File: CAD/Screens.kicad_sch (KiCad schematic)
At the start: 2 parts, among them J7 RoundDisplay_SPI, J9 RoundDisplay_SPI_v2

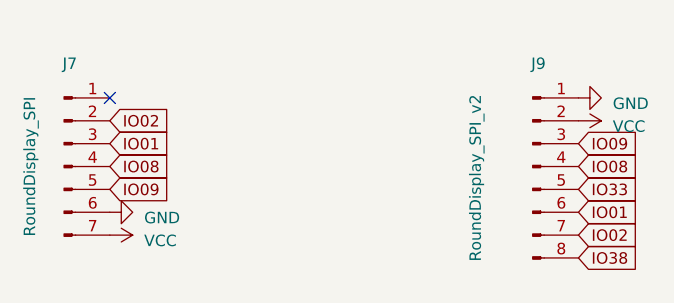
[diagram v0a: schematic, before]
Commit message: Updated pins and moar
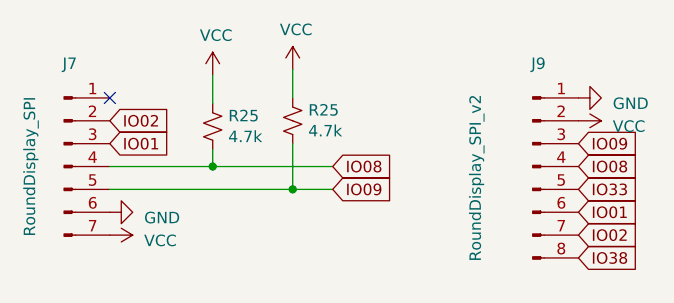
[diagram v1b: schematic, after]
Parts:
- added R25 (x2): 4.7k, BadgePirates:R_1206_3216Metric, symbol Device:R_Small_US
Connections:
- net IO08: now also R25.2
- net IO09: now also R25.2
- net VCC: now also R25.1, R25.1
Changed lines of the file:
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@@
 (kicad_sch (version 20230121) (generator eeschema)
   (paper "A4")
+  (junction (at 153.67 80.01) (diameter 0) (color 0 0 0 0)
+  )
+  (junction (at 144.78 77.47) (diameter 0) (color 0 0 0 0)
+  )
   (no_connect (at 133.35 69.85))
+  (wire (pts (xy 153.67 66.675) (xy 153.67 69.85))
+    (stroke (width 0) (type default))
+  )
+  (wire (pts (xy 144.78 75.565) (xy 144.78 77.47))
+    (stroke (width 0) (type default))
+  )
+  (wire (pts (xy 153.67 74.93) (xy 153.67 80.01))
+    (stroke (width 0) (type default))
+  )
+  (wire (pts (xy 144.78 67.31) (xy 144.78 70.485))
+    (stroke (width 0) (type default))
+  )
+  (wire (pts (xy 153.67 80.01) (xy 133.35 80.01))
+    (stroke (width 0) (type default))
+  )
+  (wire (pts (xy 158.115 80.01) (xy 153.67 80.01))
+    (stroke (width 0) (type default))
+  )
+  (wire (pts (xy 144.78 77.47) (xy 133.35 77.47))
+    (stroke (width 0) (type default))
+  )
+  (wire (pts (xy 158.115 77.47) (xy 144.78 77.47))
+    (stroke (width 0) (type default))
+  )
   (global_label "IO02" (shape input) (at 133.35 72.39 0) (fields_autoplaced)
     (effects (font (size 1.27 1.27)) (justify left))
@@
     )
   )
-  (global_label "IO08" (shape input) (at 133.35 77.47 0) (fields_autoplaced)
-    (effects (font (size 1.27 1.27)) (justify left))
-    (property "Intersheetrefs" "${INTERSHEET_REFS}" (at 139.9559 77.47 0)
+  (global_label "IO08" (shape input) (at 158.115 77.47 0) (fields_autoplaced)
+    (effects (font (size 1.27 1.27)) (justify left))
+    (property "Intersheetrefs" "${INTERSHEET_REFS}" (at 164.7209 77.47 0)
       (effects (font (size 1.27 1.27)) (justify left) hide)
     )
@@
     )
   )
-  (global_label "IO09" (shape input) (at 133.35 80.01 0) (fields_autoplaced)
-    (effects (font (size 1.27 1.27)) (justify left))
-    (property "Intersheetrefs" "${INTERSHEET_REFS}" (at 139.9559 80.01 0)
+  (global_label "IO09" (shape input) (at 158.115 80.01 0) (fields_autoplaced)
+    (effects (font (size 1.27 1.27)) (justify left))
+    (property "Intersheetrefs" "${INTERSHEET_REFS}" (at 164.7209 80.01 0)
       (effects (font (size 1.27 1.27)) (justify left) hide)
     )
@@
         (path "/76a22395-5d2d-4f66-8191-432f65fdc4ac/7bbc5ee4-a356-48de-a261-211ab35ec87b"
           (reference "#PWR068") (unit 1)
+        )
+      )
+    )
+  )
+  (symbol (lib_id "power:VCC") (at 144.78 67.31 0) (unit 1)
+    (in_bom yes) (on_board yes) (dnp no)
+    (property "Reference" "#PWR027" (at 144.78 71.12 0)
+      (effects (font (size 1.27 1.27)) hide)
+    )
+    (property "Value" "VCC" (at 145.161 62.9158 0)
+      (effects (font (size 1.27 1.27)))
+    )
+    (property "Footprint" "" (at 144.78 67.31 0)
+      (effects (font (size 1.27 1.27)) hide)
+    )
+    (property "Datasheet" "" (at 144.78 67.31 0)
+      (effects (font (size 1.27 1.27)) hide)
+    )
+    (pin "1")
+    (instances
+      (project "ProjectNeoRogue"
+        (path "/76a22395-5d2d-4f66-8191-432f65fdc4ac"
+          (reference "#PWR027") (unit 1)
+        )
+        (path "/76a22395-5d2d-4f66-8191-432f65fdc4ac/7bbc5ee4-a356-48de-a261-211ab35ec87b"
+          (reference "#PWR028") (unit 1)
         )
       )
@@
     )
   )
+  (symbol (lib_id "Device:R_Small_US") (at 153.67 72.39 0) (unit 1)
+    (in_bom yes) (on_board yes) (dnp no)
+    (property "Reference" "R25" (at 155.3972 71.2216 0)
+      (effects (font (size 1.27 1.27)) (justify left))
+    )
+    (property "Value" "4.7k" (at 155.3972 73.533 0)
+      (effects (font (size 1.27 1.27)) (justify left))
+    )
+    (property "Footprint" "BadgePirates:R_1206_3216Metric" (at 153.67 72.39 0)
+      (effects (font (size 1.27 1.27)) hide)
+    )
+    (property "Datasheet" "~" (at 153.67 72.39 0)
+      (effects (font (size 1.27 1.27)) hide)
+    )
+    (property "OrderURL" "" (at 153.67 72.39 0)
+      (effects (font (size 1.27 1.27)) hide)
+    )
+    (pin "1")
+    (pin "2")
+    (instances
+      (project "ProjectNeoRogue"
+        (path "/76a22395-5d2d-4f66-8191-432f65fdc4ac"
+          (reference "R25") (unit 1)
+        )
+        (path "/76a22395-5d2d-4f66-8191-432f65fdc4ac/7bbc5ee4-a356-48de-a261-211ab35ec87b"
+          (reference "R27") (unit 1)
+        )
+      )
+    )
+  )
+  (symbol (lib_id "Device:R_Small_US") (at 144.78 73.025 0) (unit 1)
+    (in_bom yes) (on_board yes) (dnp no)
+    (property "Reference" "R25" (at 146.5072 71.8566 0)
+      (effects (font (size 1.27 1.27)) (justify left))
+    )
+    (property "Value" "4.7k" (at 146.5072 74.168 0)
+      (effects (font (size 1.27 1.27)) (justify left))
+    )
+    (property "Footprint" "BadgePirates:R_1206_3216Metric" (at 144.78 73.025 0)
+      (effects (font (size 1.27 1.27)) hide)
+    )
+    (property "Datasheet" "~" (at 144.78 73.025 0)
+      (effects (font (size 1.27 1.27)) hide)
+    )
+    (property "OrderURL" "" (at 144.78 73.025 0)
+      (effects (font (size 1.27 1.27)) hide)
+    )
+    (pin "1")
+    (pin "2")
+    (instances
+      (project "ProjectNeoRogue"
+        (path "/76a22395-5d2d-4f66-8191-432f65fdc4ac"
+          (reference "R25") (unit 1)
+        )
+        (path "/76a22395-5d2d-4f66-8191-432f65fdc4ac/7bbc5ee4-a356-48de-a261-211ab35ec87b"
+          (reference "R23") (unit 1)
+        )
+      )
+    )
+  )
   (symbol (lib_name "GND_1") (lib_id "power:GND") (at 133.35 82.55 90) (unit 1)
     (in_bom yes) (on_board yes) (dnp no) (fields_autoplaced)
@@
         )
       )
+    )
+  )
+  (symbol (lib_id "power:VCC") (at 153.67 66.675 0) (unit 1)
+    (in_bom yes) (on_board yes) (dnp no)
+    (property "Reference" "#PWR027" (at 153.67 70.485 0)
+      (effects (font (size 1.27 1.27)) hide)
+    )
+    (property "Value" "VCC" (at 154.051 62.2808 0)
+      (effects (font (size 1.27 1.27)))
+    )
+    (property "Footprint" "" (at 153.67 66.675 0)
+      (effects (font (size 1.27 1.27)) hide)
+    )
+    (property "Datasheet" "" (at 153.67 66.675 0)
+      (effects (font (size 1.27 1.27)) hide)
+    )
+    (pin "1")
+    (instances
+      (project "ProjectNeoRogue"
+        (path "/76a22395-5d2d-4f66-8191-432f65fdc4ac"
+          (reference "#PWR027") (unit 1)
+        )
+        (path "/76a22395-5d2d-4f66-8191-432f65fdc4ac/7bbc5ee4-a356-48de-a261-211ab35ec87b"
+          (reference "#PWR032") (unit 1)
+        )
+      )
